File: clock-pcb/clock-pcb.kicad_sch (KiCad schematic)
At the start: 110 parts, among them IC2 MCP23018-E_MJ, J1 Conn_01x03_Pin, J11 Conn_01x06_Socket, J15 Conn_01x02_Socket, J2 oled 2, J3 Led display, J4 Led display 2, J5 Conn_01x07_Socket, J6 Conn_01x07_Socket, J7 SFV25R-2STE1HLF, J8 SFV25R-2STE1HLF, J9 Conn_01x04_Socket, U1 ESP32-C6-MINI-1-N4, U4 TPS2116DRL, U5 MCP73811T-420I-OT, U6 TPS61040DBV, U7 TLV75533PDBV, U8 AT42QT2120-MMHR, Y2 32.768KHz

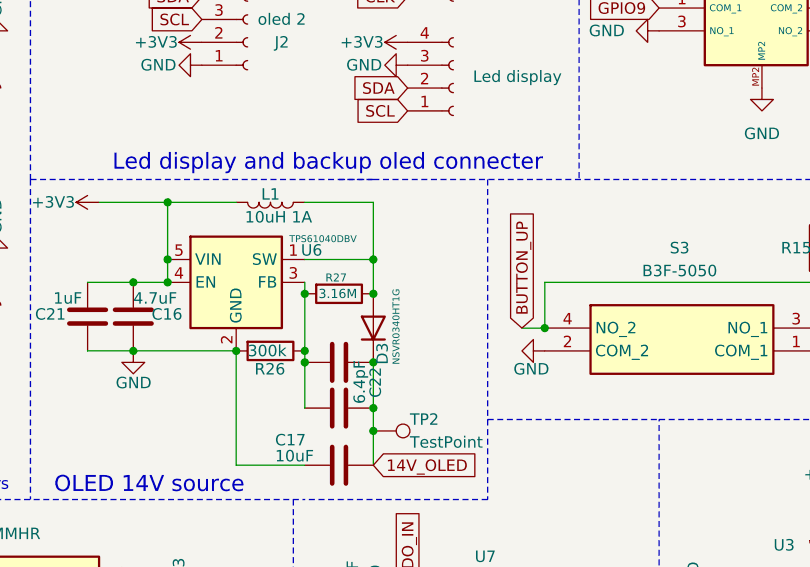
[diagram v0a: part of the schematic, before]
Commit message: not compiling yet
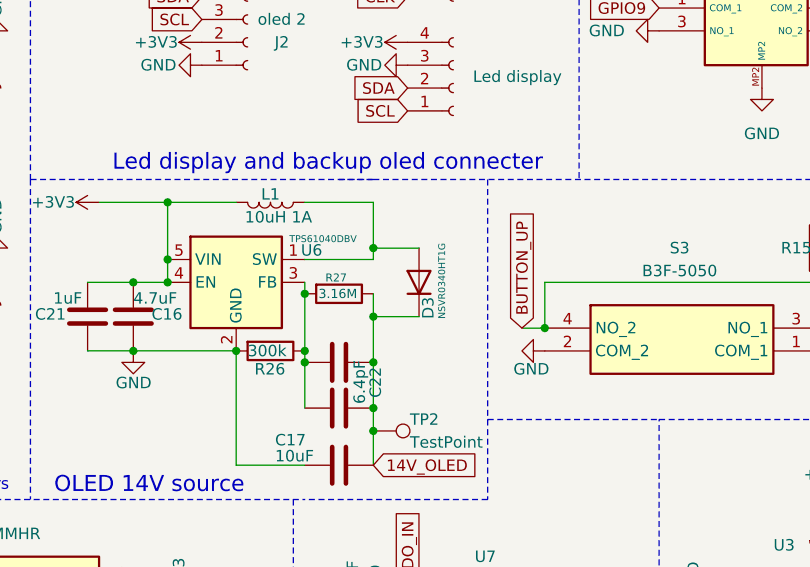
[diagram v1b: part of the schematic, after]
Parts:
- J4: footprint Connector_PinHeader_2.54mm:PinHeader_1x04_P2.54mm_Vertical -> clock:PinHeader_1x04_P2.54mm_Vertical
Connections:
- net 14V_OLED: now also R27.1
- net at D3.2 (A), L1.1, U6.1 (SW): no longer R27.1
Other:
- moved on the sheet: D3
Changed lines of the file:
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@@
 	)
 	(junction
+		(at 186.69 50.8)
+		(diameter 0)
+		(color 0 0 0 0)
+	)
+	(junction
 		(at 204.47 138.43)
 		(diameter 0)
@@
 	)
 	(junction
+		(at 186.69 58.42)
+		(diameter 0)
+		(color 0 0 0 0)
+	)
+	(junction
 		(at 163.83 54.61)
 		(diameter 0)
@@
 	)
 	(junction
-		(at 186.69 55.88)
-		(diameter 0)
-		(color 0 0 0 0)
-	)
-	(junction
 		(at 19.05 17.78)
 		(diameter 0)
@@
 	)
 	(junction
-		(at 186.69 52.07)
-		(diameter 0)
-		(color 0 0 0 0)
-	)
-	(junction
 		(at 160.02 62.23)
 		(diameter 0)
@@
 	(wire
 		(pts
+			(xy 186.69 50.8) (xy 191.77 50.8)
+		)
+		(stroke
+			(width 0)
+			(type default)
+		)
+	)
+	(wire
+		(pts
 			(xy 137.16 167.64) (xy 139.7 167.64)
 		)
@@
 	(wire
 		(pts
+			(xy 186.69 58.42) (xy 186.69 63.5)
+		)
+		(stroke
+			(width 0)
+			(type default)
+		)
+	)
+	(wire
+		(pts
 			(xy 226.06 132.08) (xy 226.06 134.62)
 		)
@@
 	(wire
 		(pts
+			(xy 186.69 50.8) (xy 186.69 52.07)
+		)
+		(stroke
+			(width 0)
+			(type default)
+		)
+	)
+	(wire
+		(pts
 			(xy 167.64 167.64) (xy 170.18 167.64)
 		)
@@
 	(wire
 		(pts
-			(xy 186.69 45.72) (xy 186.69 52.07)
+			(xy 186.69 45.72) (xy 186.69 50.8)
 		)
 		(stroke
@@
 	(wire
 		(pts
-			(xy 186.69 52.07) (xy 186.69 55.88)
-		)
-		(stroke
-			(width 0)
-			(type default)
-		)
-	)
-	(wire
-		(pts
 			(xy 179.07 55.88) (xy 179.07 54.61)
 		)
@@
 	(wire
 		(pts
+			(xy 186.69 55.88) (xy 186.69 58.42)
+		)
+		(stroke
+			(width 0)
+			(type default)
+		)
+	)
+	(wire
+		(pts
 			(xy 26.67 129.54) (xy 26.67 137.16)
 		)
@@
 		)
 	)
+	(wire
+		(pts
+			(xy 191.77 58.42) (xy 186.69 58.42)
+		)
+		(stroke
+			(width 0)
+			(type default)
+		)
+	)
 	(polyline
 		(pts
@@
 	(symbol
 		(lib_id "Device:D")
-		(at 186.69 59.69 90)
+		(at 191.77 54.61 90)
 		(unit 1)
 		(exclude_from_sim no)
@@
 		(dnp no)
 		(property "Reference" "D3"
-			(at 187.706 63.754 0)
+			(at 192.786 58.674 0)
 			(effects
 				(font
@@
 		)
 		(property "Value" "NSVR0340HT1G"
-			(at 189.23 63.754 0)
+			(at 194.31 58.674 0)
 			(effects
 				(font
@@
 		)
 		(property "Footprint" "Diode_SMD:D_SOD-323"
-			(at 186.69 59.69 0)
+			(at 191.77 54.61 0)
 			(effects
 				(font
@@
 		)
 		(property "Datasheet" "~"
-			(at 186.69 59.69 0)
+			(at 191.77 54.61 0)
 			(effects
 				(font
@@
 		)
 		(property "Description" "Diode"
-			(at 186.69 59.69 0)
+			(at 191.77 54.61 0)
 			(effects
 				(font
@@
 		)
 		(property "Sim.Device" "D"
-			(at 186.69 59.69 0)
+			(at 191.77 54.61 0)
 			(effects
 				(font
@@
 		)
 		(property "Sim.Pins" "1=K 2=A"
-			(at 186.69 59.69 0)
+			(at 191.77 54.61 0)
 			(effects
 				(font
@@
 			)
 		)
-		(property "Footprint" "Connector_PinHeader_2.54mm:PinHeader_1x04_P2.54mm_Vertical"
+		(property "Footprint" "clock:PinHeader_1x04_P2.54mm_Vertical"
 			(at 195.58 20.32 0)
 			(effects
